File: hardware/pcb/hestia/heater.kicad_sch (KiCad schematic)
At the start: 19 parts, among them Q1 FDS8876, SW2 SW_Push_Open, U10 INA826

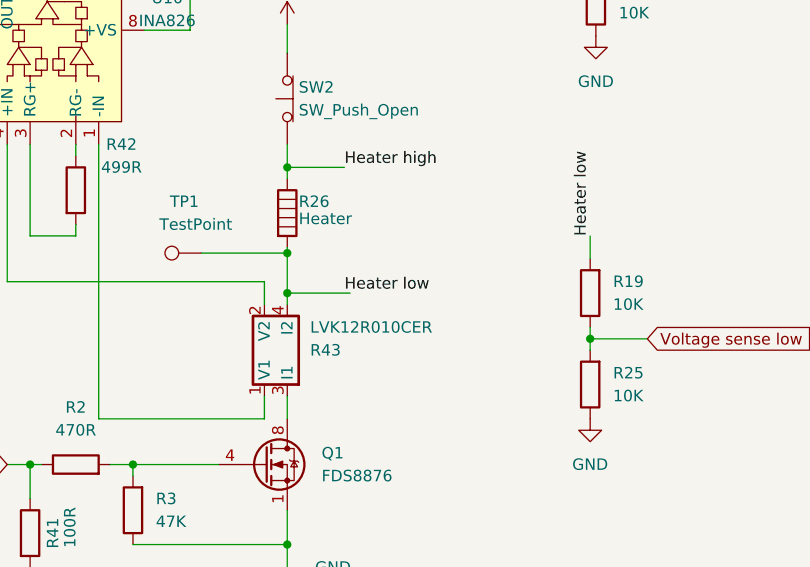
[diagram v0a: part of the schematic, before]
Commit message: changes
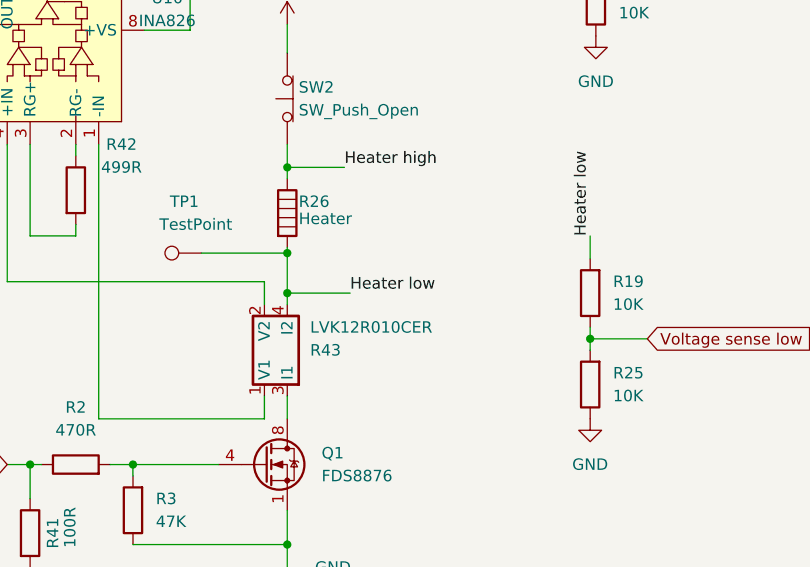
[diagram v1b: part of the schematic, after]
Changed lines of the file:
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@@
     (effects (font (size 1.27 1.27)) (justify left bottom))
   )
-  (label "Heater low" (at 135.89 103.505 0)
+  (label "Heater low" (at 136.525 103.505 0)
     (effects (font (size 1.27 1.27)) (justify left bottom))
   )
